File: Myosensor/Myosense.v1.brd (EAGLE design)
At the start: 41.9 x 58.1 mm, 26 parts, among them IC1 LM358N, IC2 LM358N, IC3 LM358N

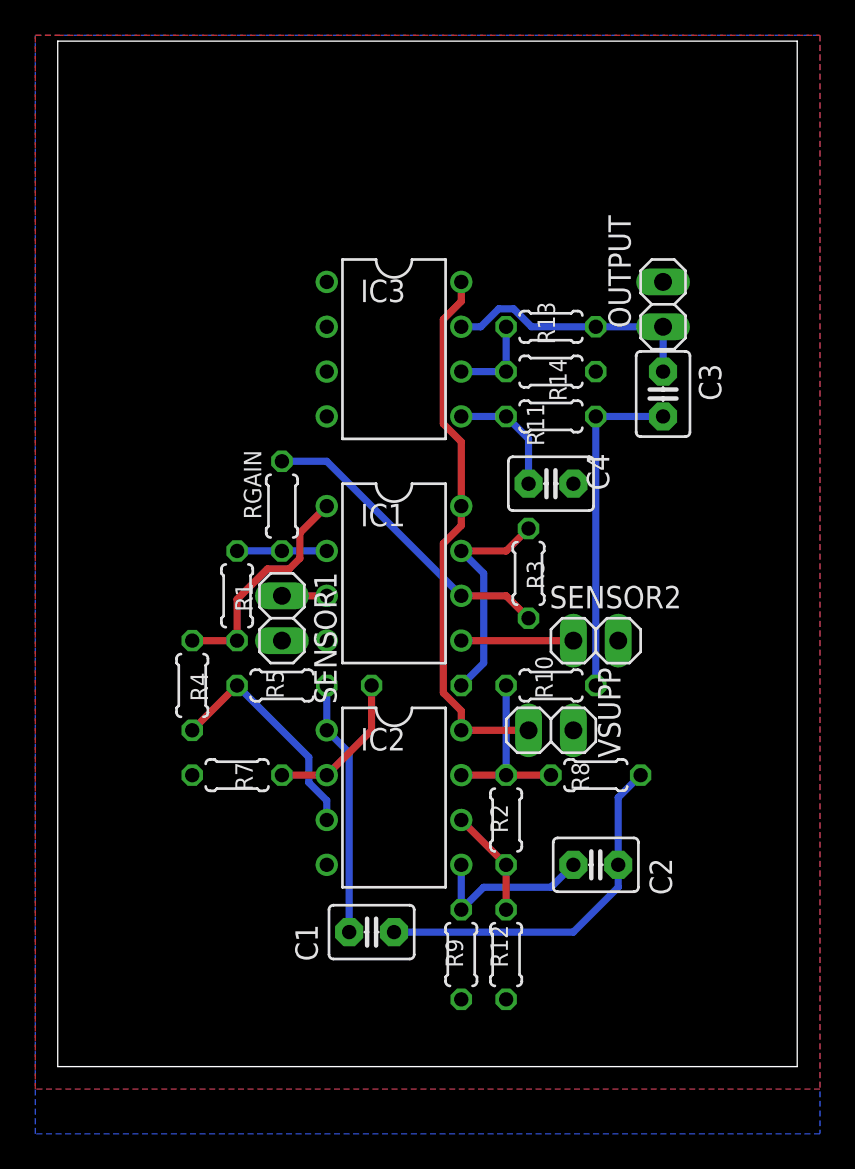
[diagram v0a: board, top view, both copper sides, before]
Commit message: Updated myosensor
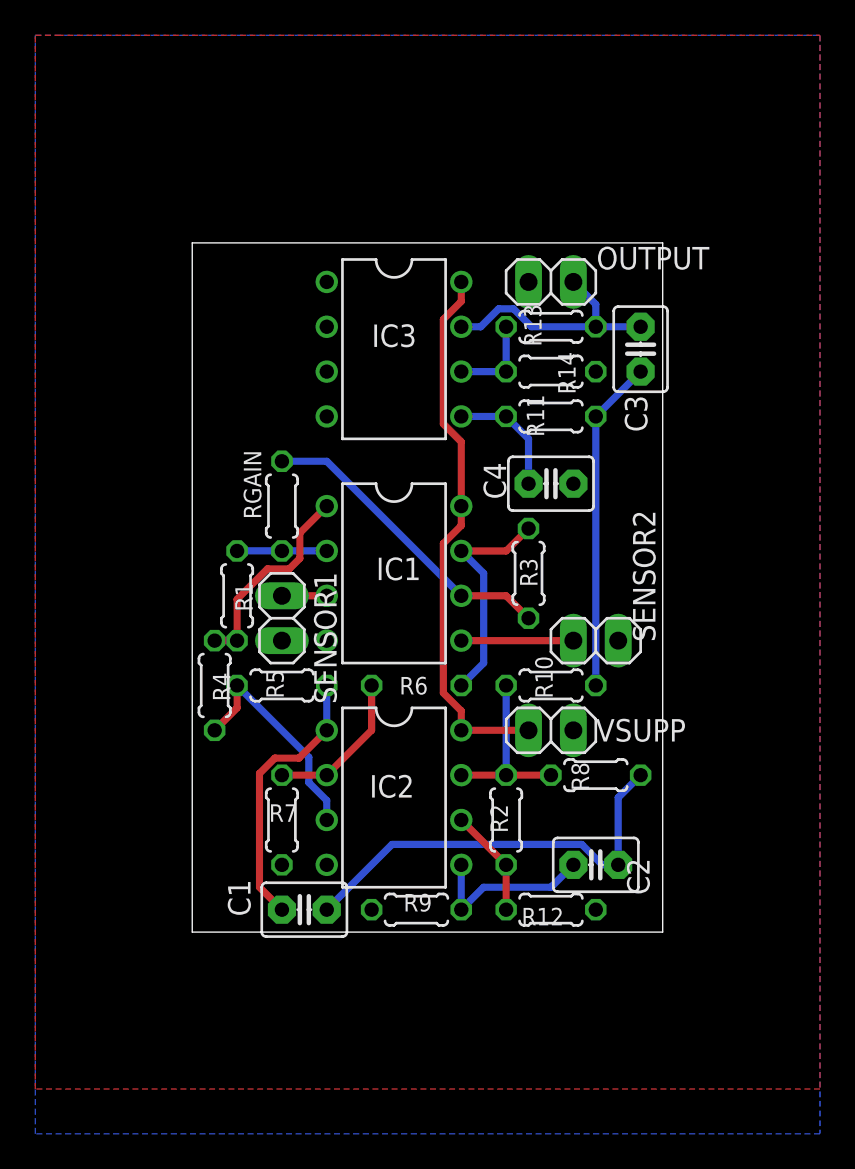
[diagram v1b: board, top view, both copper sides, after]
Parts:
- moved OUTPUT 6.48 mm to (27.9, 44.5), turned to 180 degrees
- moved C1 4.02 mm to (14.0, 8.89)
- moved R12 3.59 mm to (27.9, 8.89), turned to 180 degrees
- moved R7 3.59 mm to (12.7, 14.0), turned to 270 degrees
- moved R9 3.59 mm to (20.3, 8.89), turned to 0 degrees
- moved C3 2.84 mm to (33.0, 40.6)
- moved R4 1.27 mm to (8.89, 21.6)
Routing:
- net N$10: track 20.6 -> 24.1 mm
- net N$1: track 13.0 -> 11.7 mm
- net N$7: track 14.5 -> 15.6 mm
- net N$17: track 14.8 -> 14.1 mm
- net N$4: track 13.3 -> 12.8 mm
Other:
- board size 41.9 x 58.1 mm -> 26.7 x 39 mm
